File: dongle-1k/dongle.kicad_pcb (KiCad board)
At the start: 6 copper layers, 14 x 12 mm, 24 parts, among them U1 NRF52833-QDAA-R7, U2 TSC4A 160GF-WZ 016, U3 XL-1010RGBC-WS2812B, X1 XL7EL89CKI-111YLC-32M

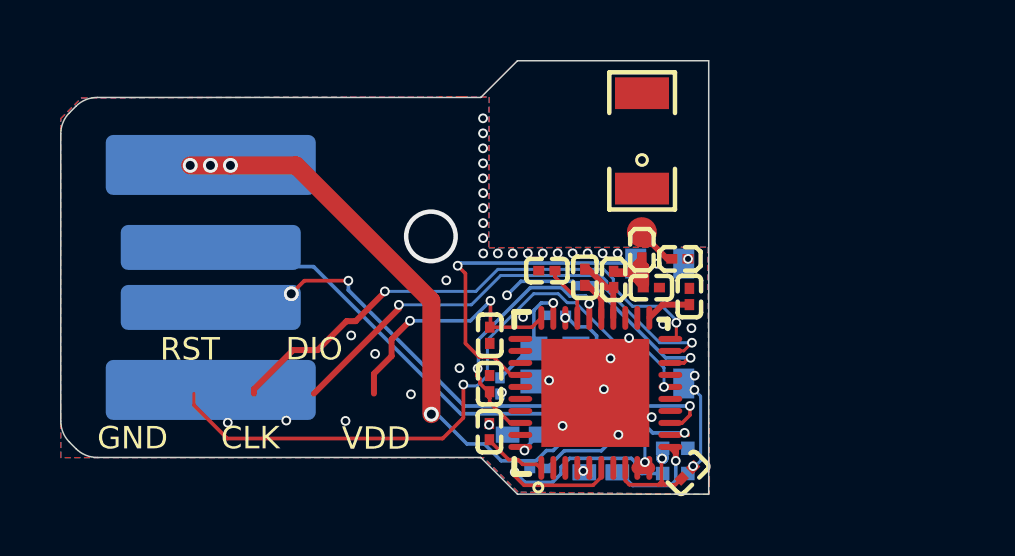
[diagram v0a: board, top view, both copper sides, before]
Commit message: feat: rev10 hardware
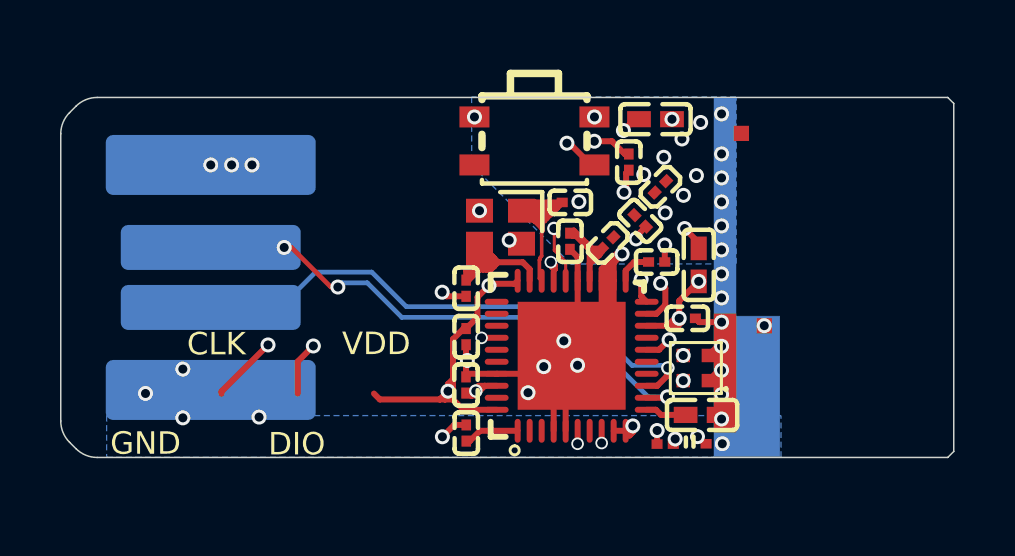
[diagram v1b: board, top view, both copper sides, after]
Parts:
- removed L1: LQP03TN6N2H02D, easyeda2kicad:L0201
- removed L2: LQP03HQ4N0B02D, easyeda2kicad:L0201
- added L4: LQP03HQ2N2H02D, easyeda2kicad:L0201, F.Cu at (196.4, 83.1)
- A1: value KH-3216-A35 -> ~; footprint easyeda2kicad:ANT-SMD-2_L3.2-W1.6-C504002 -> mifa:mifa-2.4ghz-fr4-2.0mm
- C10, C13, C14, C15, C3, C7, C8, U2, U3, X1: moved to F.Cu
- moved C7 10.7 mm to (196.3, 80.8)
- moved A1 10.2 mm to (206.0, 81.1), turned to -90 degrees
- moved C13 8.12 mm to (197.7, 85.7), turned to 90 degrees
- moved U2 7.38 mm to (192.2, 81.6), turned to 180 degrees
- moved C10 5.93 mm to (198.2, 91.7)
- moved X1 4.94 mm to (191.1, 84.4)
- moved C5 4.53 mm to (195.4, 82.3), turned to 90 degrees
- moved C8 3.88 mm to (197.8, 90.7), turned to 0 degrees
- moved C14 3.79 mm to (193.4, 83.6), turned to 0 degrees
- moved C3 3.57 mm to (197.3, 87.5), turned to 180 degrees
- moved C15 3.45 mm to (189.9, 86.5)
- moved U3 3.17 mm to (197.6, 89.1)
- moved C4 2.26 mm to (195.7, 84.2), turned to 135 degrees
- moved C1 1.58 mm to (196.3, 85.6), turned to 180 degrees
- moved U1 1.47 mm to (193.5, 88.7)
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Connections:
- A1 pad 2: unconnected-(A1-Pad2) -> GND
- C13 pad 1: Net-(C13-Pad1) -> VDD
- C3 pad 2: Net-(C3-Pad2) -> VDD
- C6 pad 2: Net-(C6-Pad2) -> VDD
- U1 pad 18: Net-(C3-Pad2) -> VDD
- U1 pad 30: Net-(C6-Pad2) -> VDD
- U1 pad 40: Net-(C13-Pad1) -> VDD
- U3 pad 1: unconnected-(U3-DOUT-Pad1) -> GND
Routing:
- net GND: track 10.3 -> 35.9 mm, vias 47 -> 45
- net MCU_RESET: track 21.5 -> 0.85 mm, vias 2 -> 1
- net VDD: track 3.99 -> 17.3 mm, vias 1 -> 7
- net Net-(C6-Pad2): track 8.62 -> 0.00 mm, vias 2 -> 0
- net MCU_XC2: track 4.14 -> 12.2 mm, vias 1 -> 0
- net MCU_XC1: track 3.17 -> 10.3 mm, vias 1 -> 0
- net Net-(U1-DEC3): track 1.89 -> 7.87 mm, vias 0 -> 2
- net Net-(C3-Pad2): track 4.98 -> 0.00 mm, vias 1 -> 0
- net RGBD: track 9.40 -> 5.14 mm, vias 1 -> 2
- net Net-(C4-Pad2): track 6.19 -> 2.06 mm
- net USB_D_N: track 18.8 -> 15.7 mm, vias 1 -> 3
- net Net-(U1-ANT): track 2.23 -> 5.17 mm
- net USB_VBUS: track 27.2 -> 30.1 mm, vias 5 -> 6
- net DEC46: track 8.45 -> 11.0 mm
- net Net-(U1-DECUSB): track 3.52 -> 1.37 mm, vias 1 -> 0
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- added copper zone on In2.Cu, net VDD
- added copper zone on In3.Cu, net VDD
- removed copper zone on F.Cu, net GND
- removed copper zone on In2.Cu, net GND
- removed copper zone on In3.Cu, net GND
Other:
- board size 14 x 12 mm -> 15.8 x 12 mm
- board text added: "EFOG.TECH"
- board text added: "rev 2"
- board text removed: "RST"
- board text removed: "rev 1"
